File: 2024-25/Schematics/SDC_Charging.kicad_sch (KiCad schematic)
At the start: 34 parts, among them K2 GV24 1BAX, K4 P115 BDA, K5 1462043-3, K6 1462043-3, K7 1462043-3, M1 SI2101A-TP, M2 SI2101A-TP, Q3 PJA3412_R1_00001, Q4 PJA3412_R1_00001, SW1 3491, SW2 84-5330.0020, SW4 UPCP012ALS2, U1 HEF4049BT,653, U2 HEF4049BT,653, U3 TLV6703DDCR

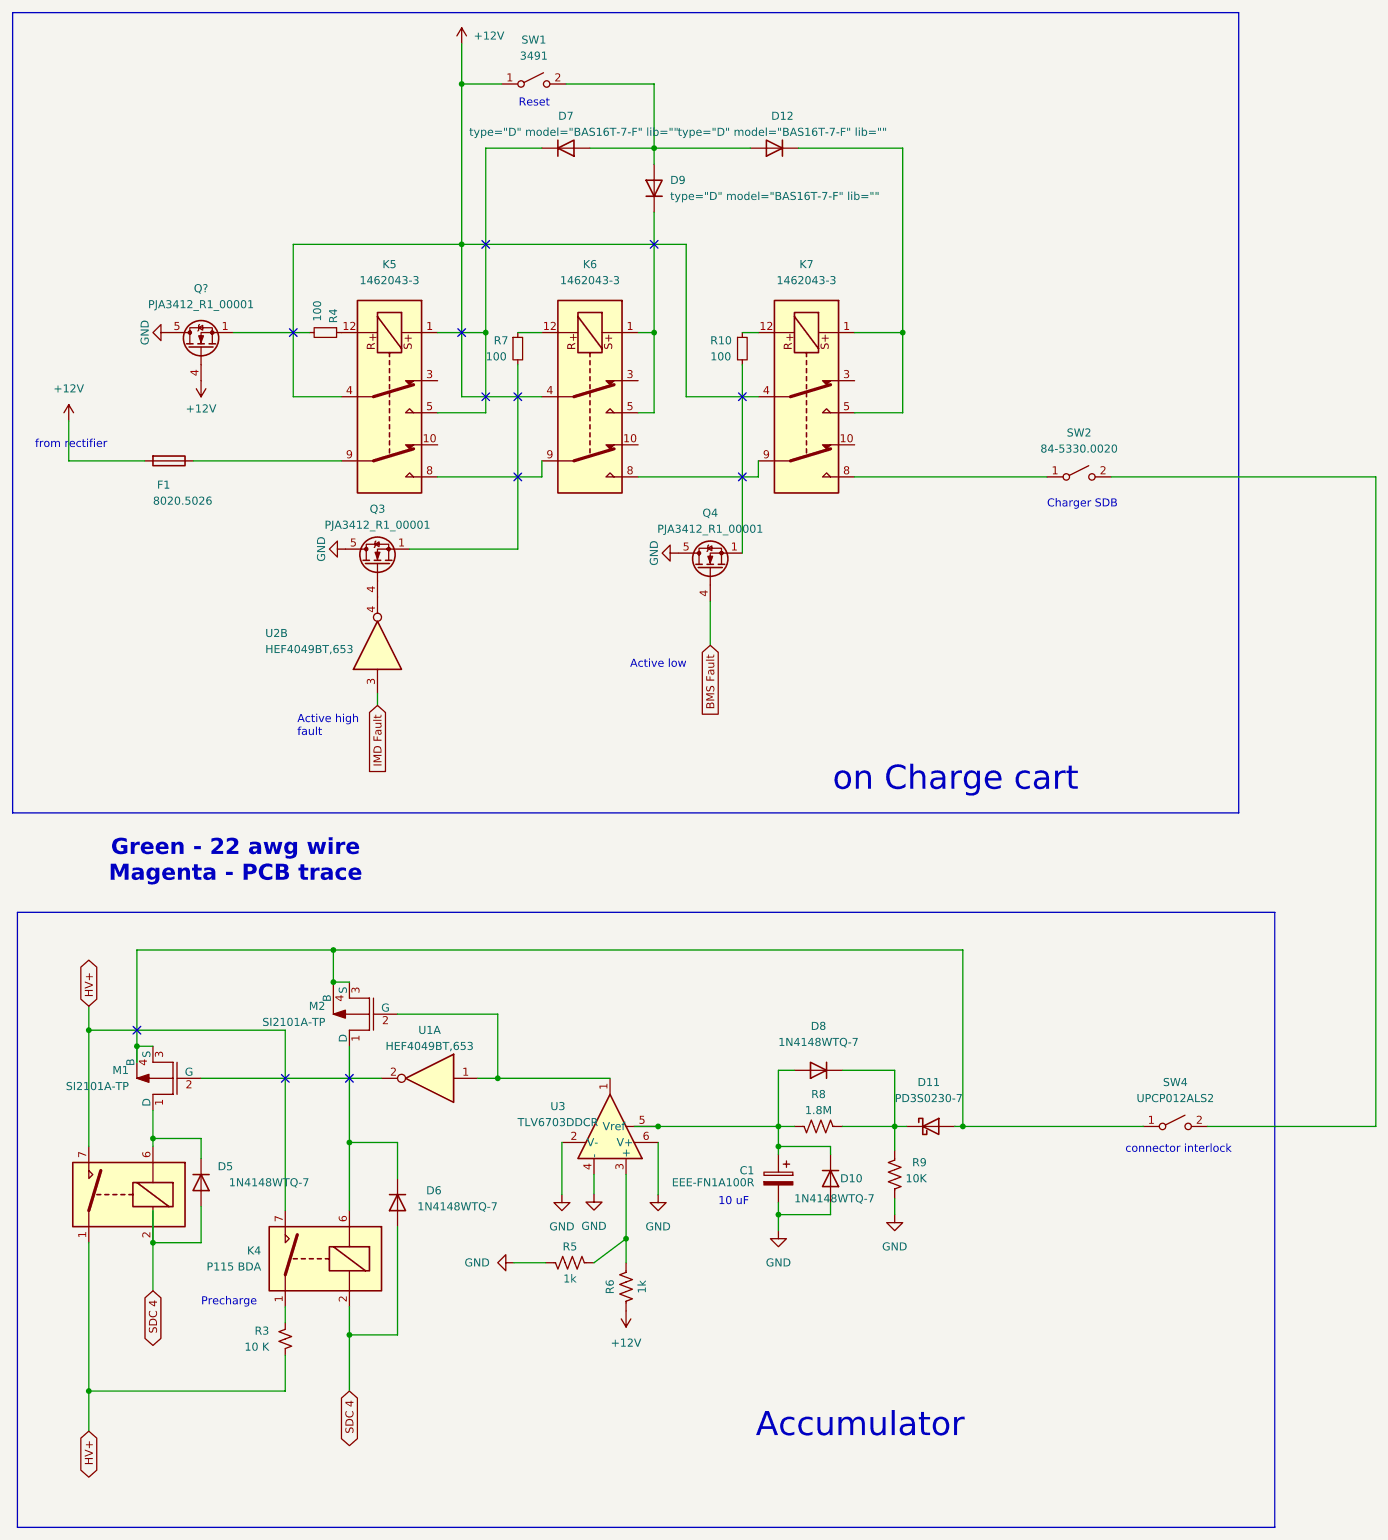
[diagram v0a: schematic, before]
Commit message: ESF fixes
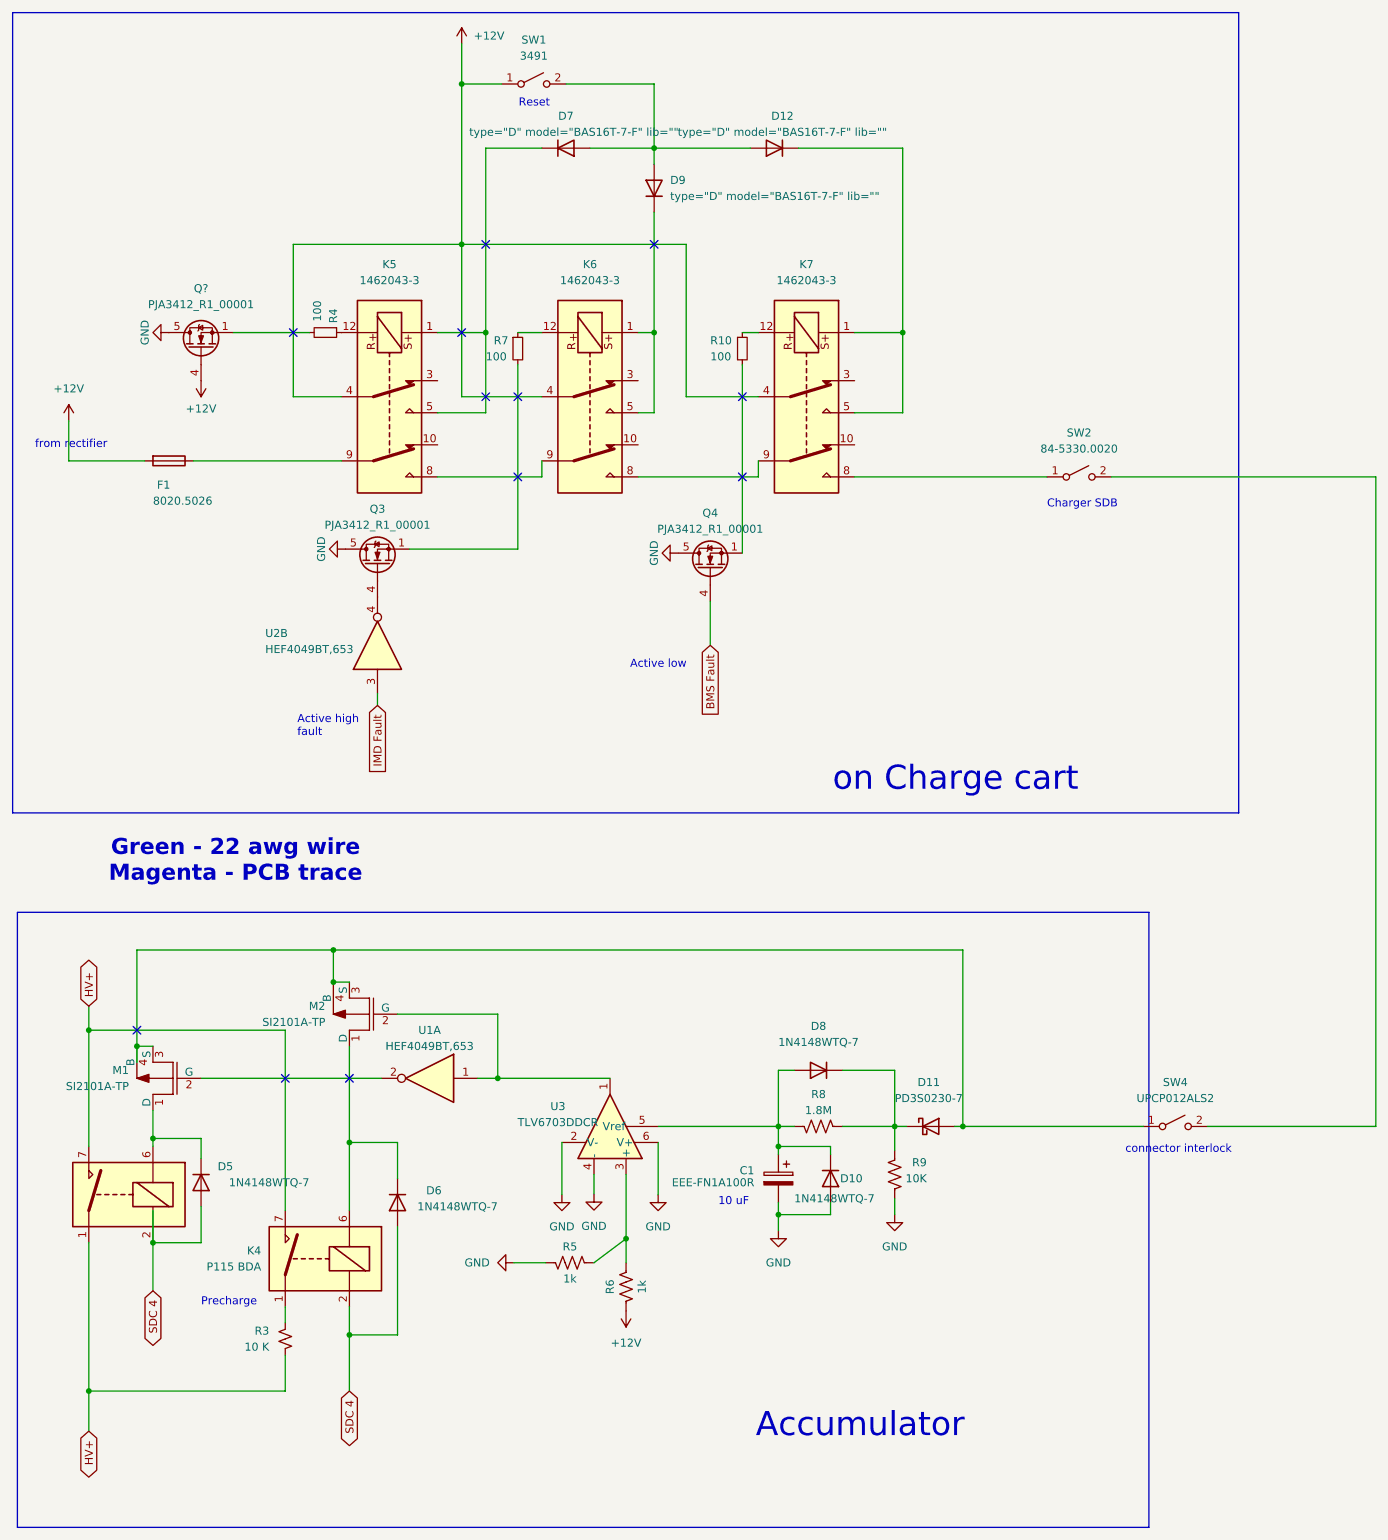
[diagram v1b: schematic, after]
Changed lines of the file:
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@@
-	)
-	(junction
-		(at 133.985 203.835)
-		(diameter 0)
-		(color 0 0 0 0)
 	)
 	(junction
@@
 	(wire
 		(pts
-			(xy 133.985 203.835) (xy 130.175 203.835)
-		)
-		(stroke
-			(width 0)
-			(type default)
-		)
-	)
-	(wire
-		(pts
 			(xy 182.245 175.895) (xy 82.55 175.895)
 		)
@@
 			(width 0)
 			(type default)
+			(color 132 0 132 1)
 		)
 	)
@@
 			(width 0)
 			(type default)
+			(color 132 0 132 1)
 		)
 	)
@@
 			(width 0)
 			(type default)
+			(color 132 0 132 1)
 		)
 	)
@@
 	(rectangle
 		(start 32.512 169.926)
-		(end 231.648 267.335)
-		(stroke
-			(width 0)
+		(end 211.709 267.335)
+		(stroke
+			(width 0)
